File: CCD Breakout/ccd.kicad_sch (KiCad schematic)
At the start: 17 parts, among them U1 CCD, U5 74HC541PW_118

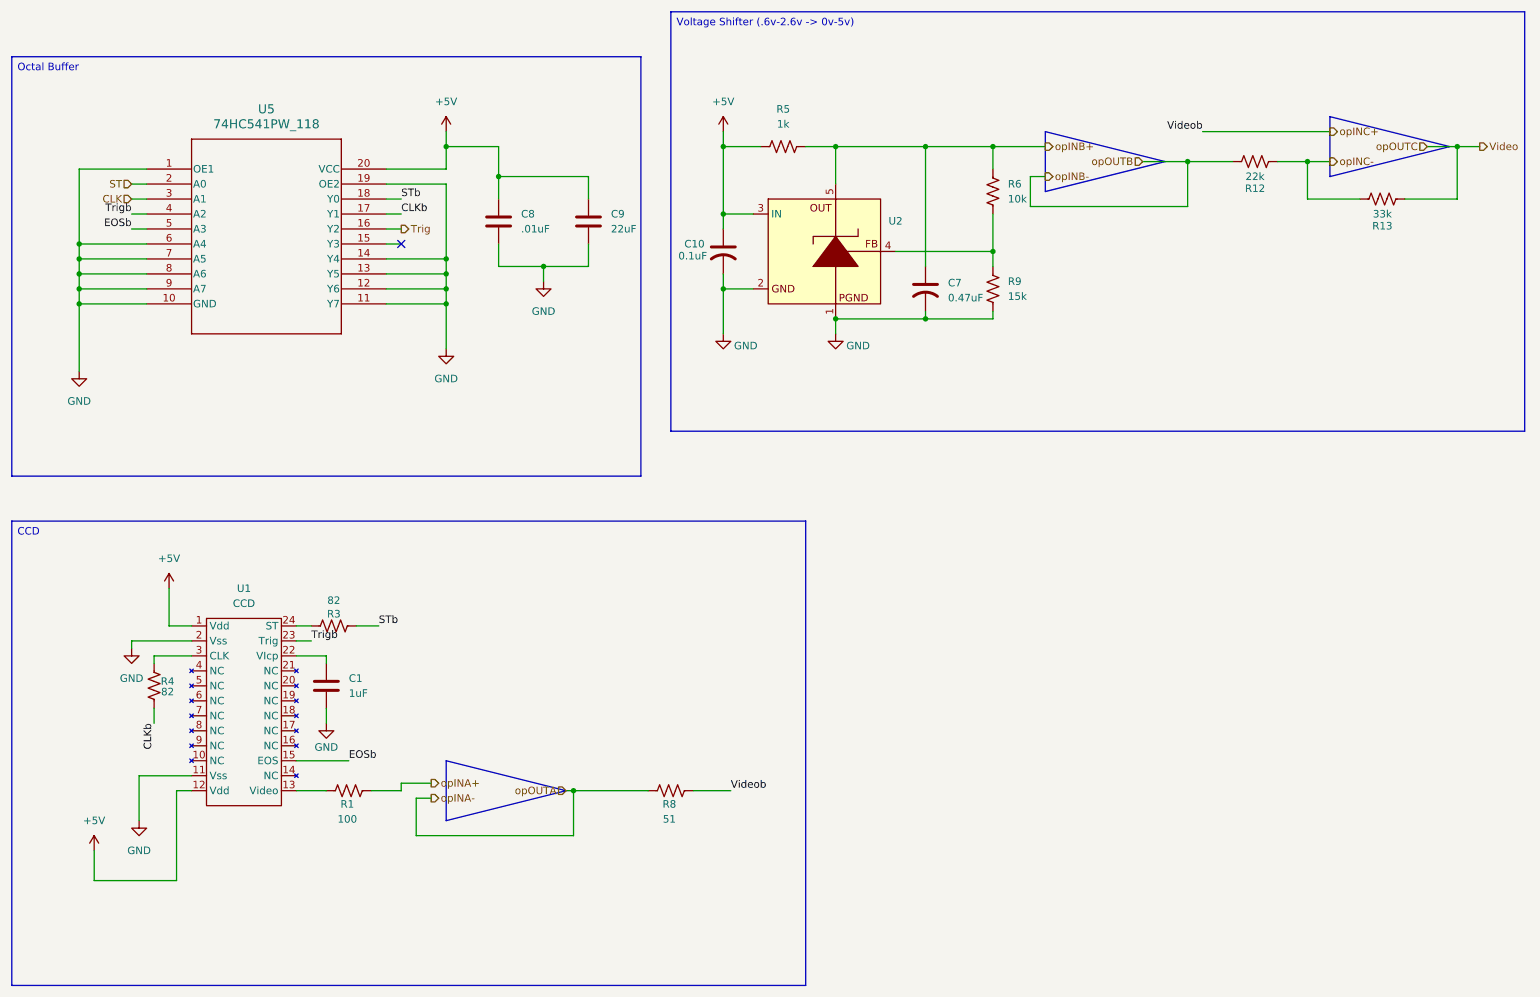
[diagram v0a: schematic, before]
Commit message: Miscellaneous schematic fixes
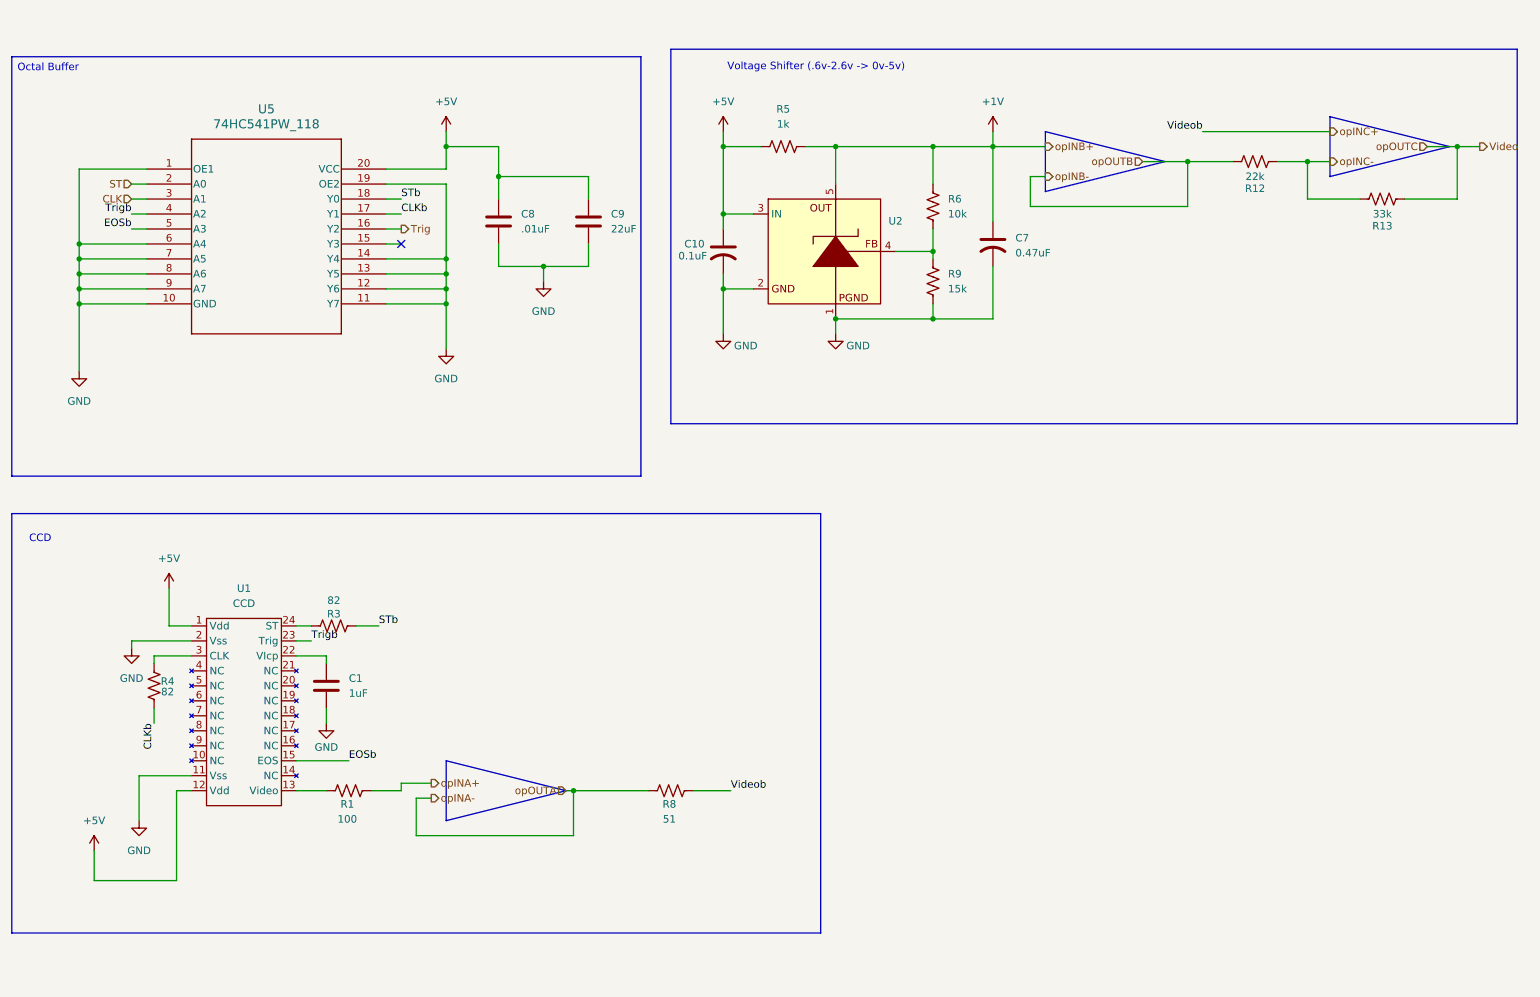
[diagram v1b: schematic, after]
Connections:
- net opINB+ renamed +1V
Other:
- note added: "CCD"
- note added: "Voltage Shifter (.6v-2.6v -> 0v-5v)"
- moved on the sheet: C7, R6, R9
